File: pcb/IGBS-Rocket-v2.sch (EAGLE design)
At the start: 159 parts, among them Q1 BC817, Q2 ENC-03, U1 STM32H750VBT6, U2 LD1085D2M-R, U3 LD1085D2M-R, U4 LM317SX/NOPB, U5 MICROSD, U6 ESP-12E/F, U8 LP324DRG4, U9 MCP6V51T-E/MS, Y1 24MHz

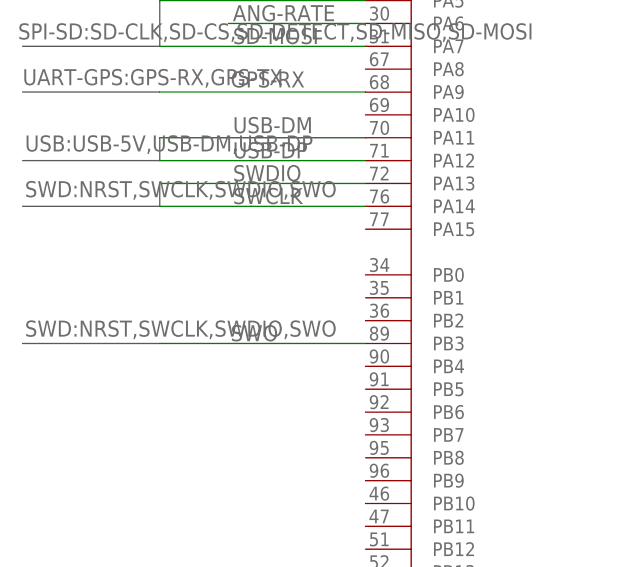
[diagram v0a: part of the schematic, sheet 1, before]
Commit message: PCB CAD - update
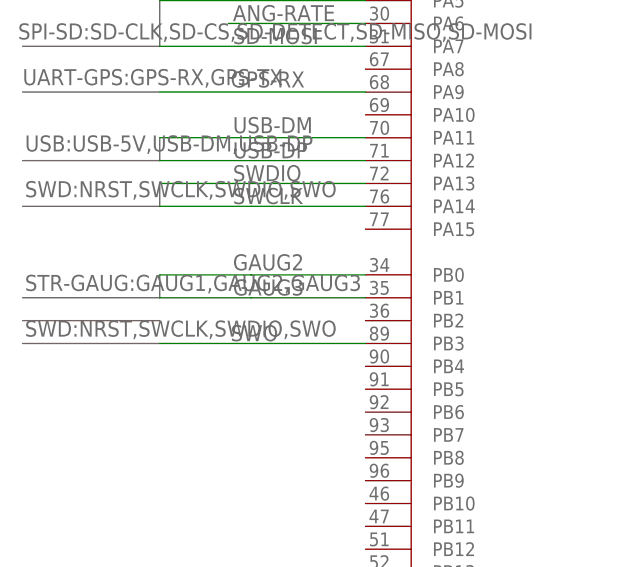
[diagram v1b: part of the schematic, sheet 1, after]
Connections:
- net GAUG2: now also U1A.PB0
- net GAUG3: now also U1A.PB1
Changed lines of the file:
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@@
+</segment>
+</bus>
+<bus name="STR-GAUG:GAUG1,GAUG2,GAUG3">
+<segment>
+<wire x1="22.86" y1="83.82" x2="22.86" y2="81.28" width="0.762" layer="92"/>
+<wire x1="22.86" y1="81.28" x2="7.62" y2="81.28" width="0.762" layer="92"/>
+<label x="7.874" y="82.042" size="1.778" layer="95"/>
+</segment>
+</bus>
+<bus name="GAUG3">
+<segment>
+<wire x1="7.62" y1="78.74" x2="22.86" y2="78.74" width="0.762" layer="92"/>
 </segment>
 </bus>
@@
 </segment>
 </net>
+<net name="GAUG2" class="0">
+<segment>
+<wire x1="22.86" y1="83.82" x2="33.02" y2="83.82" width="0.1524" layer="91"/>
+<wire x1="33.02" y1="83.82" x2="45.72" y2="83.82" width="0.1524" layer="91"/>
+<label x="30.988" y="84.328" size="1.778" layer="95"/>
+<pinref part="U1" gate="A" pin="PB0"/>
+</segment>
+</net>
+<net name="GAUG3" class="0">
+<segment>
+<wire x1="22.86" y1="81.28" x2="33.02" y2="81.28" width="0.1524" layer="91"/>
+<wire x1="33.02" y1="81.28" x2="45.72" y2="81.28" width="0.1524" layer="91"/>
+<label x="30.988" y="81.534" size="1.778" layer="95"/>
+<pinref part="U1" gate="A" pin="PB1"/>
+</segment>
+</net>
